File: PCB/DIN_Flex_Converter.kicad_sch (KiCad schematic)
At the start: 36 parts, among them IC1 ZXTR2005Z-13, J1 Screw_Terminal_01x04, J2 Screw_Terminal_01x04, J3 Conn_01x04_Socket, J4 Conn_02x06_Top_Bottom, J5 Conn_02x06_Top_Bottom, U1 74HC04

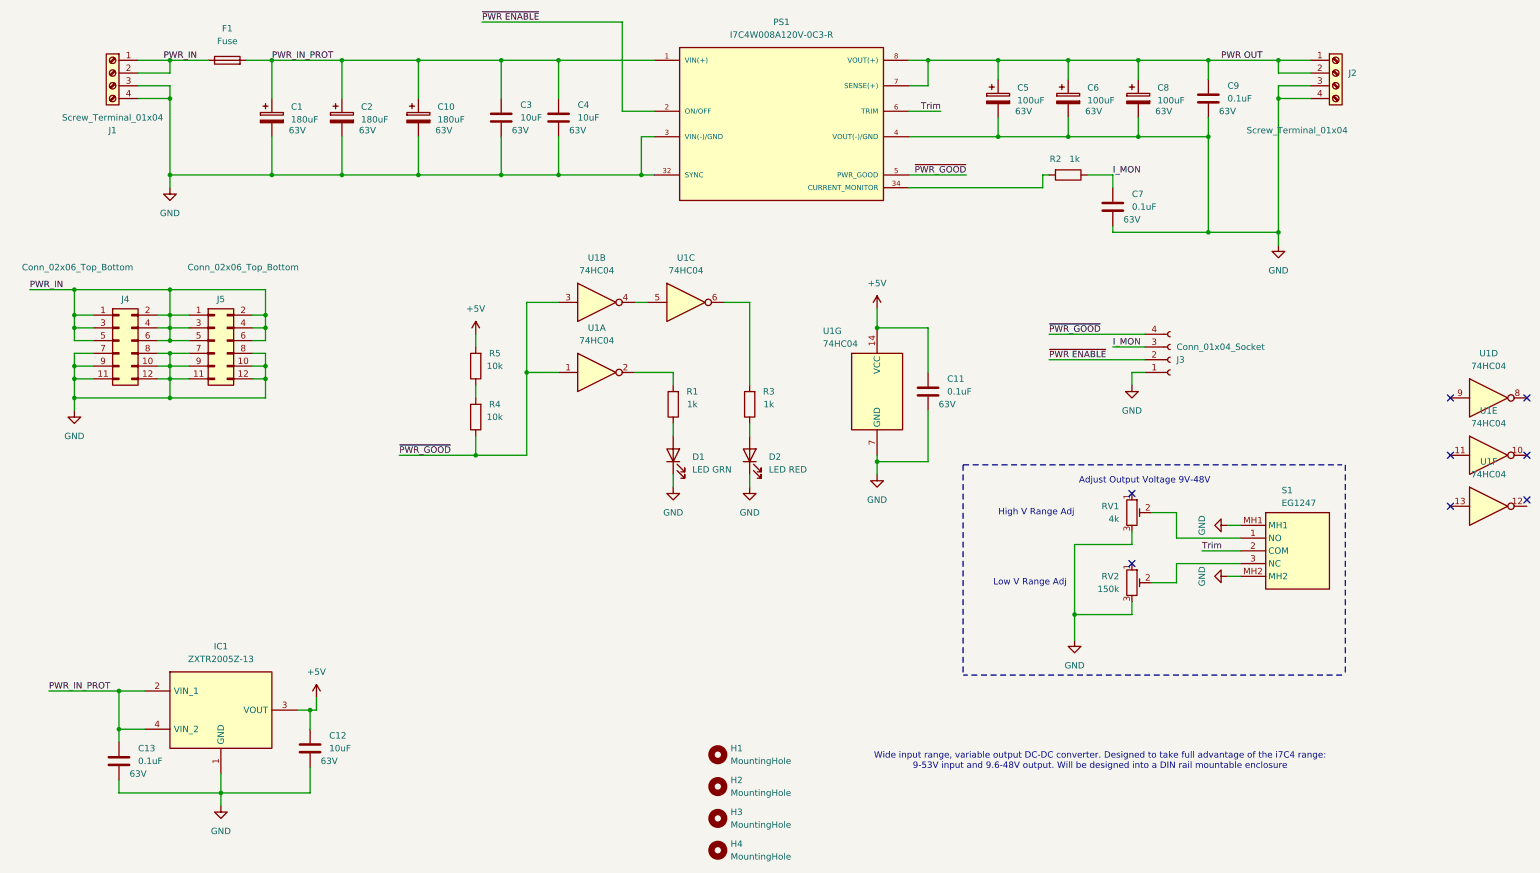
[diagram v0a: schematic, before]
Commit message: PCB Finalized and manufacturing files generated
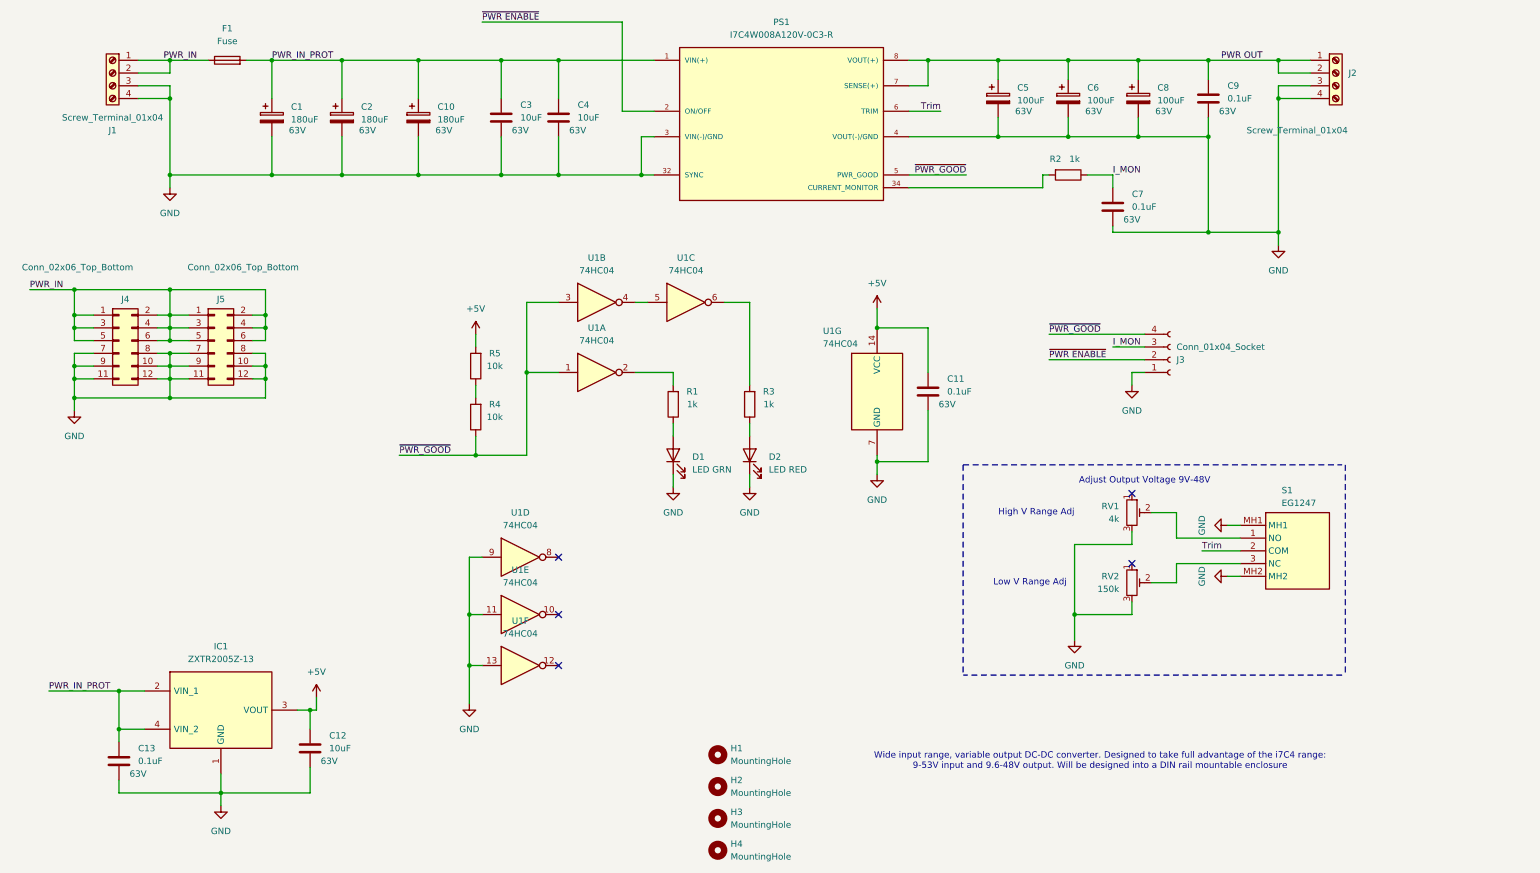
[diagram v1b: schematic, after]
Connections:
- net GND: now also U1.11, U1.13, U1.9
- no-connect marks 8 -> 5
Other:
- moved on the sheet: U1D, U1E, U1F
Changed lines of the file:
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@@
 	)
 	(junction
+		(at 106.68 152.4)
+		(diameter 0)
+		(color 0 0 0 0)
+	)
+	(junction
 		(at 140.97 54.61)
 		(diameter 0)
@@
 	)
 	(junction
+		(at 106.68 142.24)
+		(diameter 0)
+		(color 0 0 0 0)
+	)
+	(junction
 		(at 96.52 31.75)
 		(diameter 0)
@@
 	)
 	(no_connect
-		(at 238.76 132.08)
-	)
-	(no_connect
-		(at 317.5 99.06)
-	)
-	(no_connect
-		(at 317.5 119.38)
-	)
-	(no_connect
-		(at 238.76 118.11)
+		(at 124.46 130.81)
 	)
 	(no_connect
-		(at 302.26 120.65)
+		(at 238.76 132.08)
 	)
 	(no_connect
-		(at 302.26 99.06)
+		(at 124.46 142.24)
 	)
 	(no_connect
-		(at 317.5 110.49)
+		(at 124.46 152.4)
 	)
 	(no_connect
-		(at 302.26 110.49)
+		(at 238.76 118.11)
 	)
 	(wire
@@
 	(wire
 		(pts
+			(xy 106.68 142.24) (xy 109.22 142.24)
+		)
+		(stroke
+			(width 0)
+			(type default)
+		)
+	)
+	(wire
+		(pts
 			(xy 41.91 165.1) (xy 36.83 165.1)
 		)
@@
 	(wire
 		(pts
+			(xy 106.68 142.24) (xy 106.68 152.4)
+		)
+		(stroke
+			(width 0)
+			(type default)
+		)
+	)
+	(wire
+		(pts
 			(xy 50.8 85.09) (xy 46.99 85.09)
 		)
@@
 	(wire
 		(pts
+			(xy 109.22 130.81) (xy 106.68 130.81)
+		)
+		(stroke
+			(width 0)
+			(type default)
+		)
+	)
+	(wire
+		(pts
 			(xy 74.93 177.8) (xy 57.15 177.8)
 		)
@@
 	(wire
 		(pts
+			(xy 106.68 130.81) (xy 106.68 142.24)
+		)
+		(stroke
+			(width 0)
+			(type default)
+		)
+	)
+	(wire
+		(pts
 			(xy 226.06 46.99) (xy 240.03 46.99)
 		)
@@
 	(wire
 		(pts
+			(xy 106.68 152.4) (xy 109.22 152.4)
+		)
+		(stroke
+			(width 0)
+			(type default)
+		)
+	)
+	(wire
+		(pts
 			(xy 147.32 114.3) (xy 147.32 116.84)
 		)
@@
 	(wire
 		(pts
+			(xy 106.68 152.4) (xy 106.68 160.02)
+		)
+		(stroke
+			(width 0)
+			(type default)
+		)
+	)
+	(wire
+		(pts
 			(xy 40.64 34.29) (xy 46.99 34.29)
 		)
@@
 	(symbol
 		(lib_id "74xx:74HC04")
-		(at 309.88 120.65 0)
+		(at 116.84 152.4 0)
 		(unit 6)
 		(exclude_from_sim no)
@@
 		(fields_autoplaced yes)
 		(property "Reference" "U1"
-			(at 309.88 111.76 0)
+			(at 116.84 143.51 0)
 			(effects
 				(font
@@
 		)
 		(property "Value" "74HC04"
-			(at 309.88 114.3 0)
+			(at 116.84 146.05 0)
 			(effects
 				(font
@@
 		)
 		(property "Footprint" "PSA:SOIC127P600X175-14N"
-			(at 309.88 120.65 0)
+			(at 116.84 152.4 0)
 			(effects
 				(font
@@
 		)
 		(property "Datasheet" "https://assets.nexperia.com/documents/data-sheet/74HC_HCT04.pdf"
-			(at 309.88 120.65 0)
+			(at 116.84 152.4 0)
 			(effects
 				(font
@@
 		)
 		(property "Description" "Hex Inverter"
-			(at 309.88 120.65 0)
+			(at 116.84 152.4 0)
 			(effects
 				(font
@@
 		(lib_name "GND_14")
 		(lib_id "power:GND")
+		(at 106.68 160.02 0)
+		(unit 1)
+		(exclude_from_sim no)
+		(in_bom yes)
+		(on_board yes)
+		(dnp no)
+		(fields_autoplaced yes)
+		(property "Reference" "#PWR015"
+			(at 106.68 166.37 0)
+			(effects
+				(font
+					(size 1.27 1.27)
+				)
+				(hide yes)
+			)
+		)
+		(property "Value" "GND"
+			(at 106.68 165.1 0)
+			(effects
+				(font
+					(size 1.27 1.27)
+				)
+			)
+		)
+		(property "Footprint" ""
+			(at 106.68 160.02 0)
+			(effects
+				(font
+					(size 1.27 1.27)
+				)
+				(hide yes)
+			)
+		)
+		(property "Datasheet" ""
+			(at 106.68 160.02 0)
+			(effects
+				(font
+					(size 1.27 1.27)
+				)
+				(hide yes)
+			)
+		)
+		(property "Description" ""
+			(at 106.68 160.02 0)
+			(effects
+				(font
+					(size 1.27 1.27)
+				)
+				(hide yes)
+			)
+		)
+		(pin "1"
+		)
+		(instances
+			(project "DIN_Flex_Converter"
+				(path "/e44269d9-3860-4750-a5c6-e30e8b477b13"
+					(reference "#PWR015")
+					(unit 1)
+				)
+			)
+		)
+	)
+	(symbol
+		(lib_name "GND_14")
+		(lib_id "power:GND")
 		(at 257.81 134.62 270)
 		(unit 1)
@@
 	(symbol
 		(lib_id "74xx:74HC04")
-		(at 309.88 110.49 0)
+		(at 116.84 142.24 0)
 		(unit 5)
 		(exclude_from_sim no)
@@
 		(fields_autoplaced yes)
 		(property "Reference" "U1"
-			(at 309.88 101.6 0)
+			(at 116.84 133.35 0)
 			(effects
 				(font
@@
 		)
 		(property "Value" "74HC04"
-			(at 309.88 104.14 0)
+			(at 116.84 135.89 0)
 			(effects
 				(font
@@
 		)
 		(property "Footprint" "PSA:SOIC127P600X175-14N"
-			(at 309.88 110.49 0)
+			(at 116.84 142.24 0)
 			(effects
 				(font
@@
 		)
 		(property "Datasheet" "https://assets.nexperia.com/documents/data-sheet/74HC_HCT04.pdf"
-			(at 309.88 110.49 0)
+			(at 116.84 142.24 0)
 			(effects
 				(font
@@
 		)
 		(property "Description" "Hex Inverter"
-			(at 309.88 110.49 0)
+			(at 116.84 142.24 0)
 			(effects
 				(font
@@
 	(symbol
 		(lib_id "74xx:74HC04")
-		(at 309.88 99.06 0)
+		(at 116.84 130.81 0)
 		(unit 4)
 		(exclude_from_sim no)
@@
 		(fields_autoplaced yes)
 		(property "Reference" "U1"
-			(at 309.88 90.17 0)
+			(at 116.84 121.92 0)
 			(effects
 				(font
@@
 		)
 		(property "Value" "74HC04"
-			(at 309.88 92.71 0)
+			(at 116.84 124.46 0)
 			(effects
 				(font
@@
 		)
 		(property "Footprint" "PSA:SOIC127P600X175-14N"
-			(at 309.88 99.06 0)
+			(at 116.84 130.81 0)
 			(effects
 				(font
@@
 		)
 		(property "Datasheet" "https://assets.nexperia.com/documents/data-sheet/74HC_HCT04.pdf"
-			(at 309.88 99.06 0)
+			(at 116.84 130.81 0)
 			(effects
 				(font
@@
 		)
 		(property "Description" "Hex Inverter"
-			(at 309.88 99.06 0)
+			(at 116.84 130.81 0)
 			(effects
 				(font
